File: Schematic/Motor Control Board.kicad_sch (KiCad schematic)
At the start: 0 parts

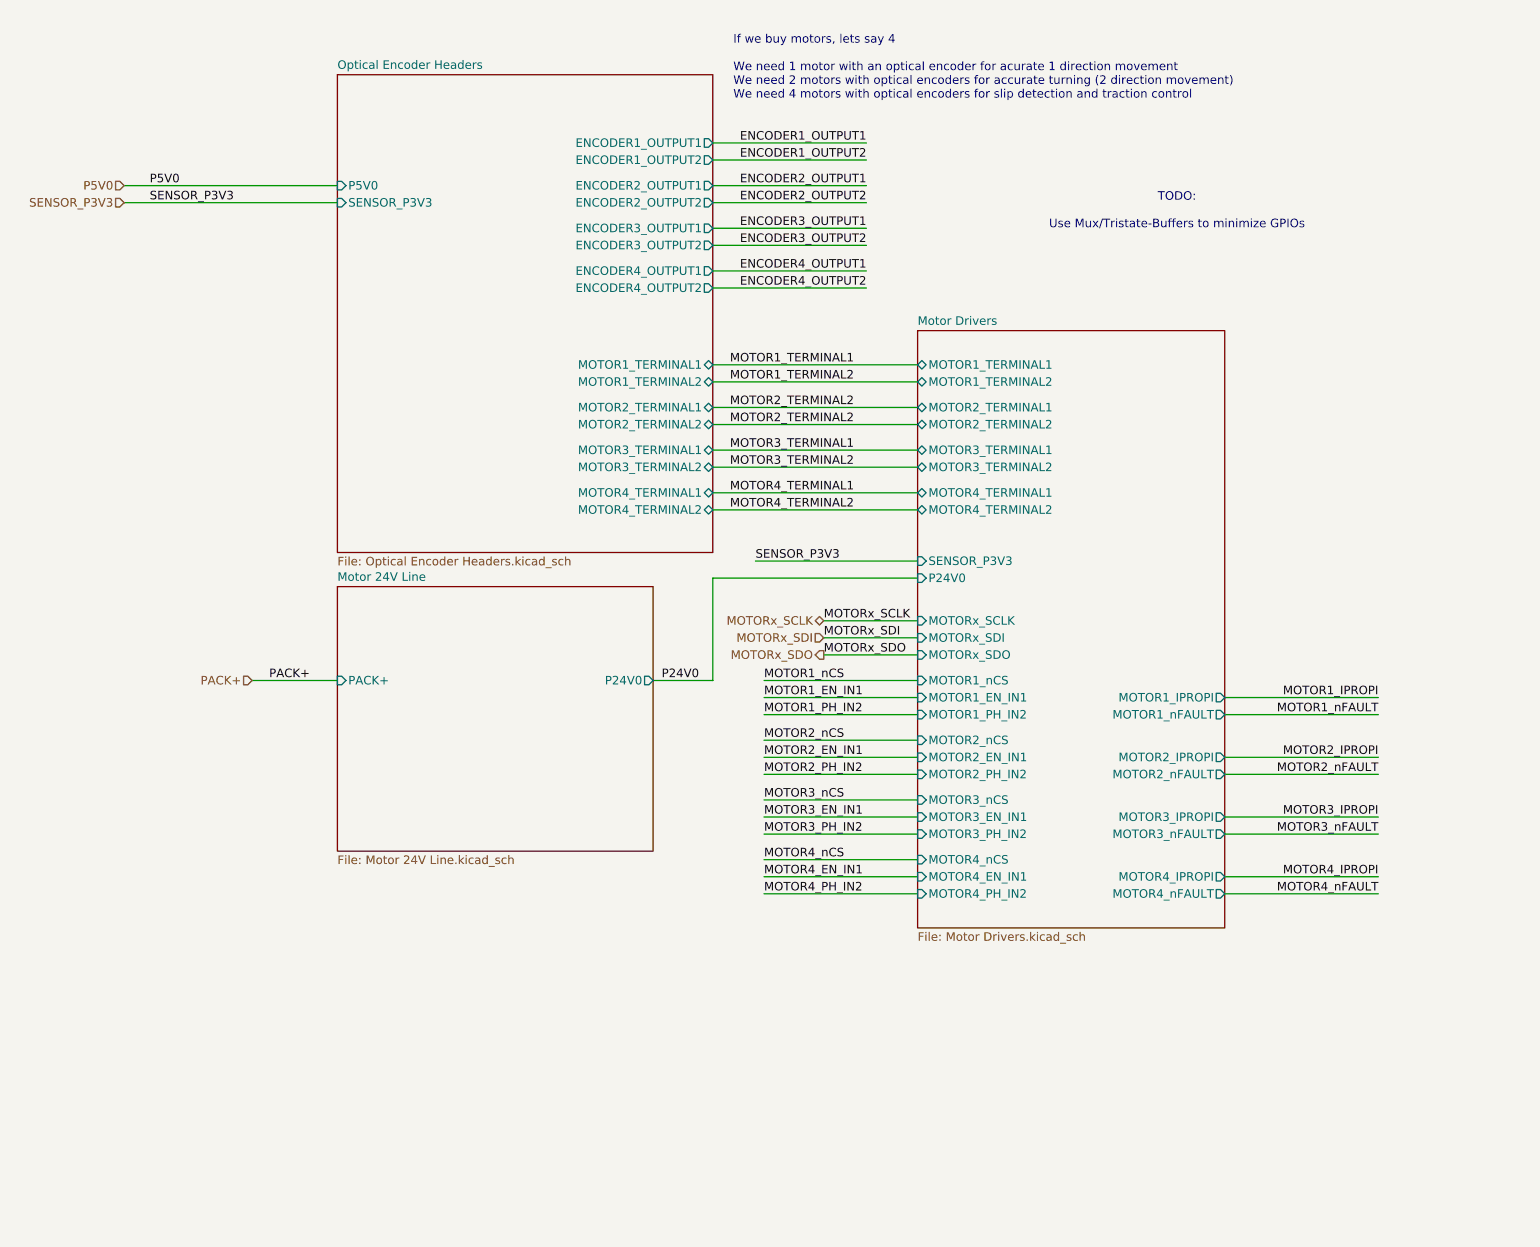
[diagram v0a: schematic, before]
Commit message: 1st Schematic Review
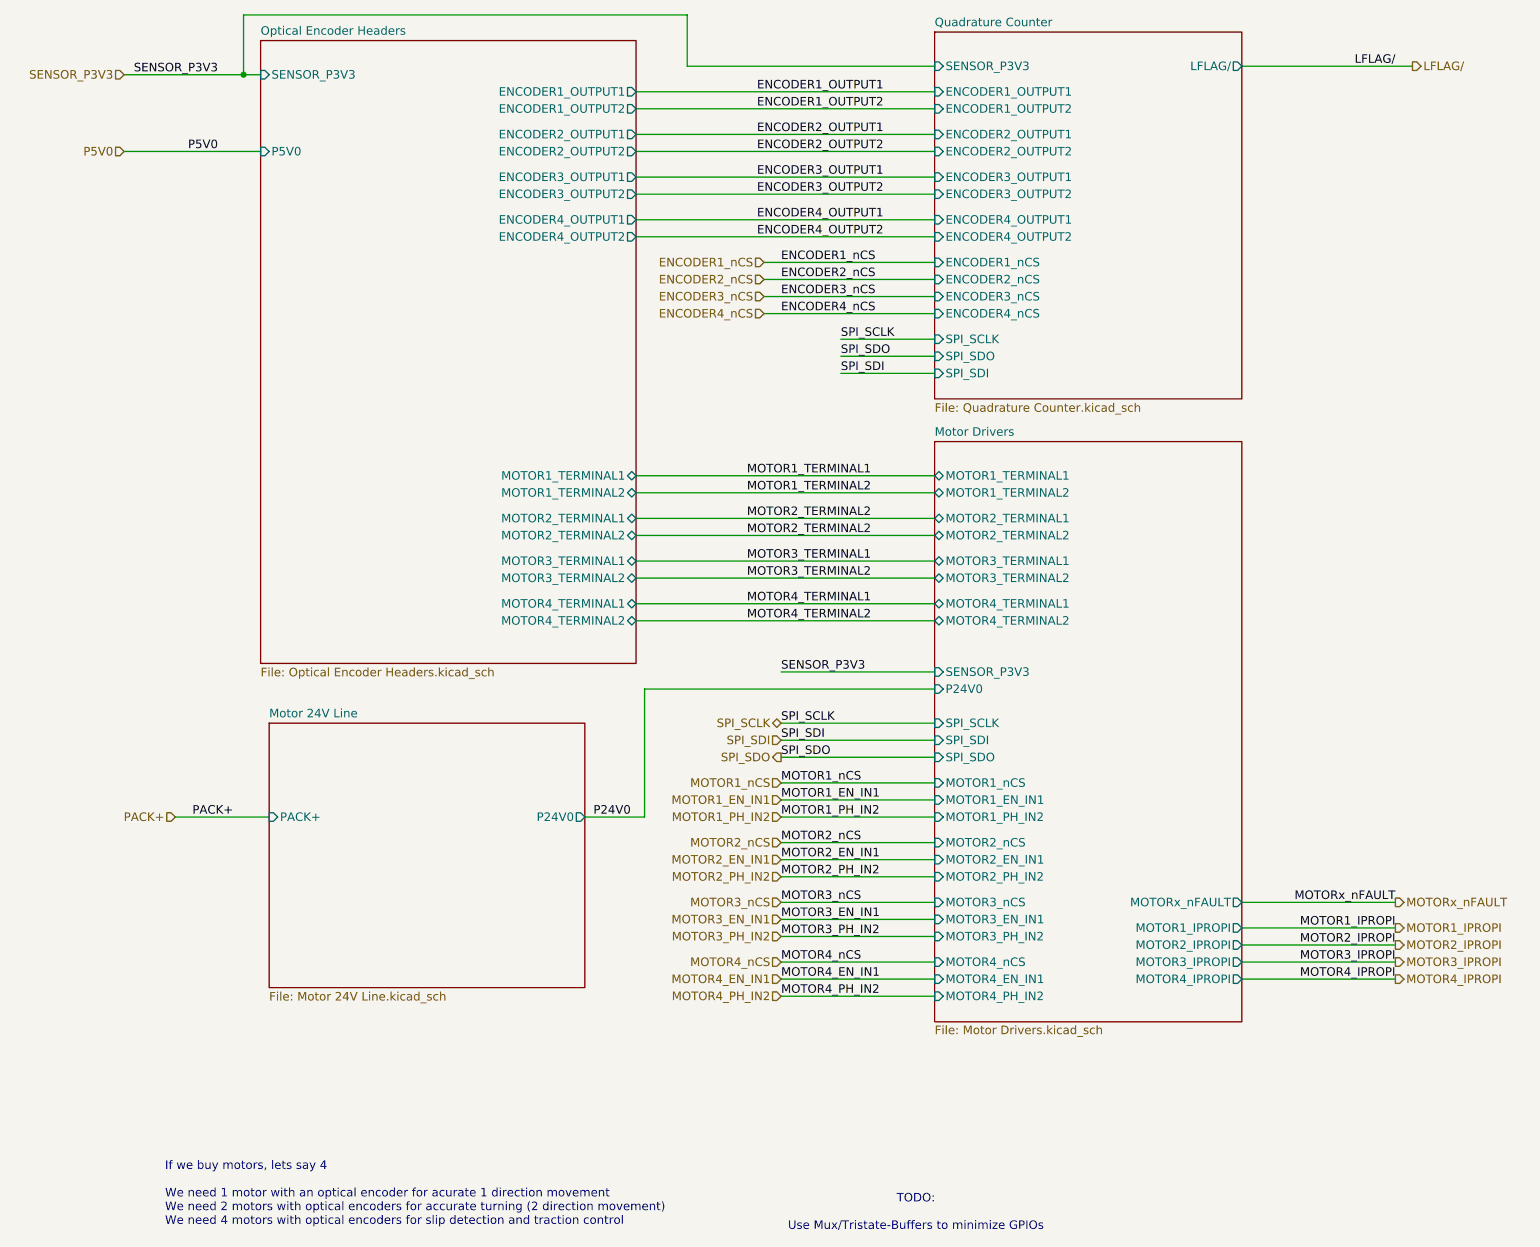
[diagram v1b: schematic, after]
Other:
- added sheet Quadrature Counter (Quadrature Counter.kicad_sch)
- sheet Motor Drivers ports: added MOTORx_nFAULT, SPI_SCLK, SPI_SDI, SPI_SDO; removed MOTOR1_nFAULT, MOTOR2_nFAULT, MOTOR3_nFAULT, MOTOR4_nFAULT, MOTORx_SCLK, MOTORx_SDI, MOTORx_SDO
